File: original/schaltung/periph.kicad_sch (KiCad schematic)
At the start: 31 parts, among them T13 SF129, T14 SS216, T15 SS216, T16 SC308

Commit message: Schönheitskorrekturen Schaltplan
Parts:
- D11: symbol RFT_Transistoren_und_Dioden:SZX21/xx -> RFT_Transistoren_und_Dioden:SZX21/xx

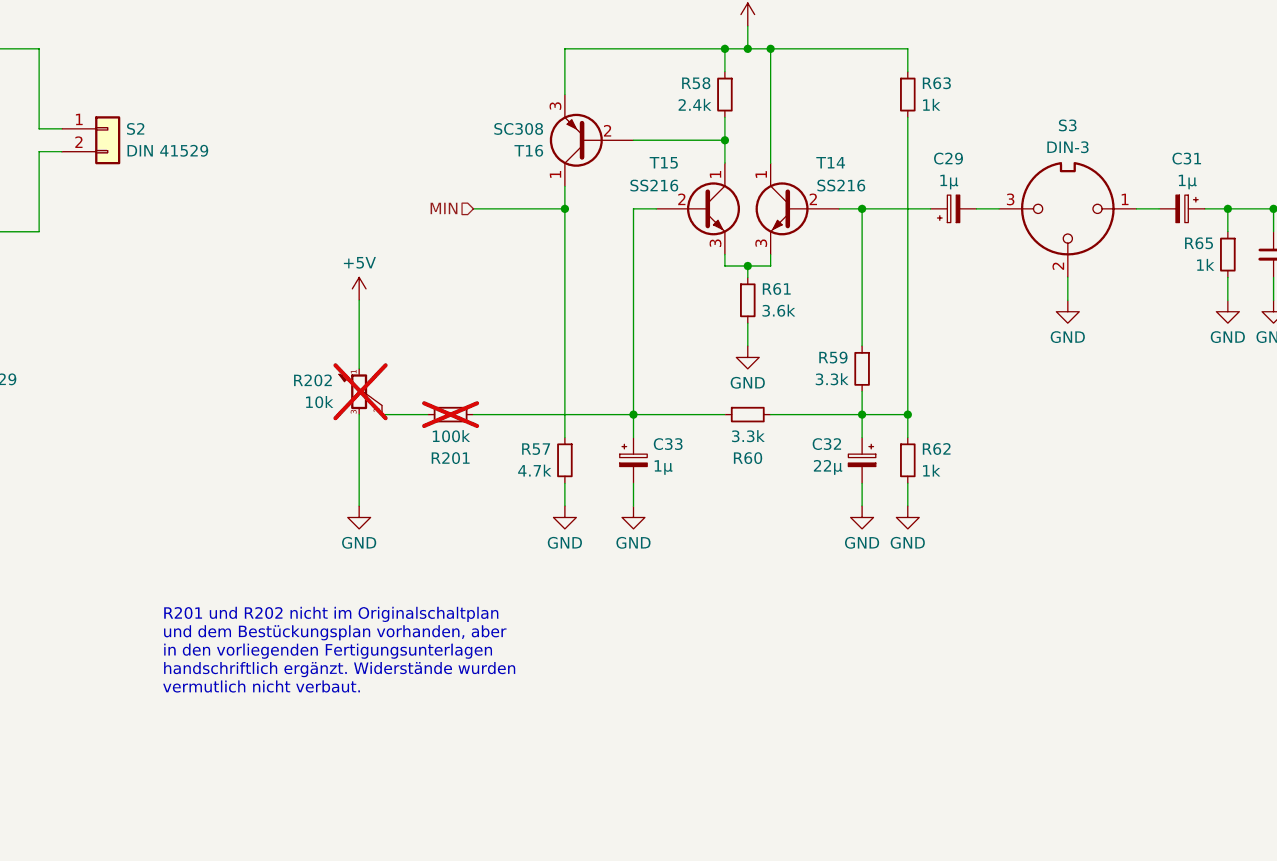
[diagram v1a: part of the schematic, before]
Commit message: Typo Schaltplan
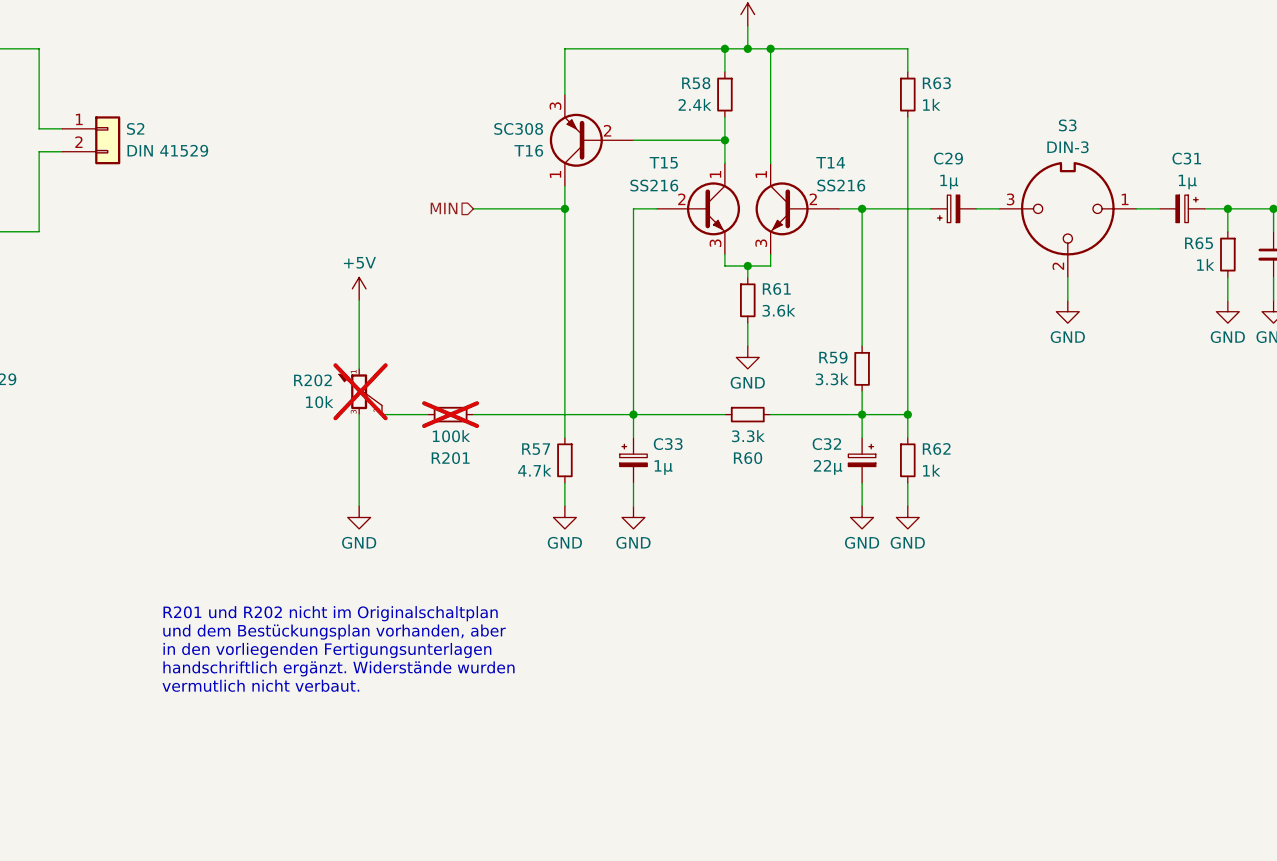
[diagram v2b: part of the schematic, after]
